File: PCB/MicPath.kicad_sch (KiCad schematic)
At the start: 53 parts, among them J301 NC3FAH, J302 Conn_01x02, J303 Conn_01x02, J304 Conn_01x02, J305 Conn_01x02, J306 NC3MAH, J307 NC3MAH, SW301 SW_SPST, SW302 SW_SPST, U301 THAT1512, U302 TMUX6236, U303 THAT1646, U304 THAT1646

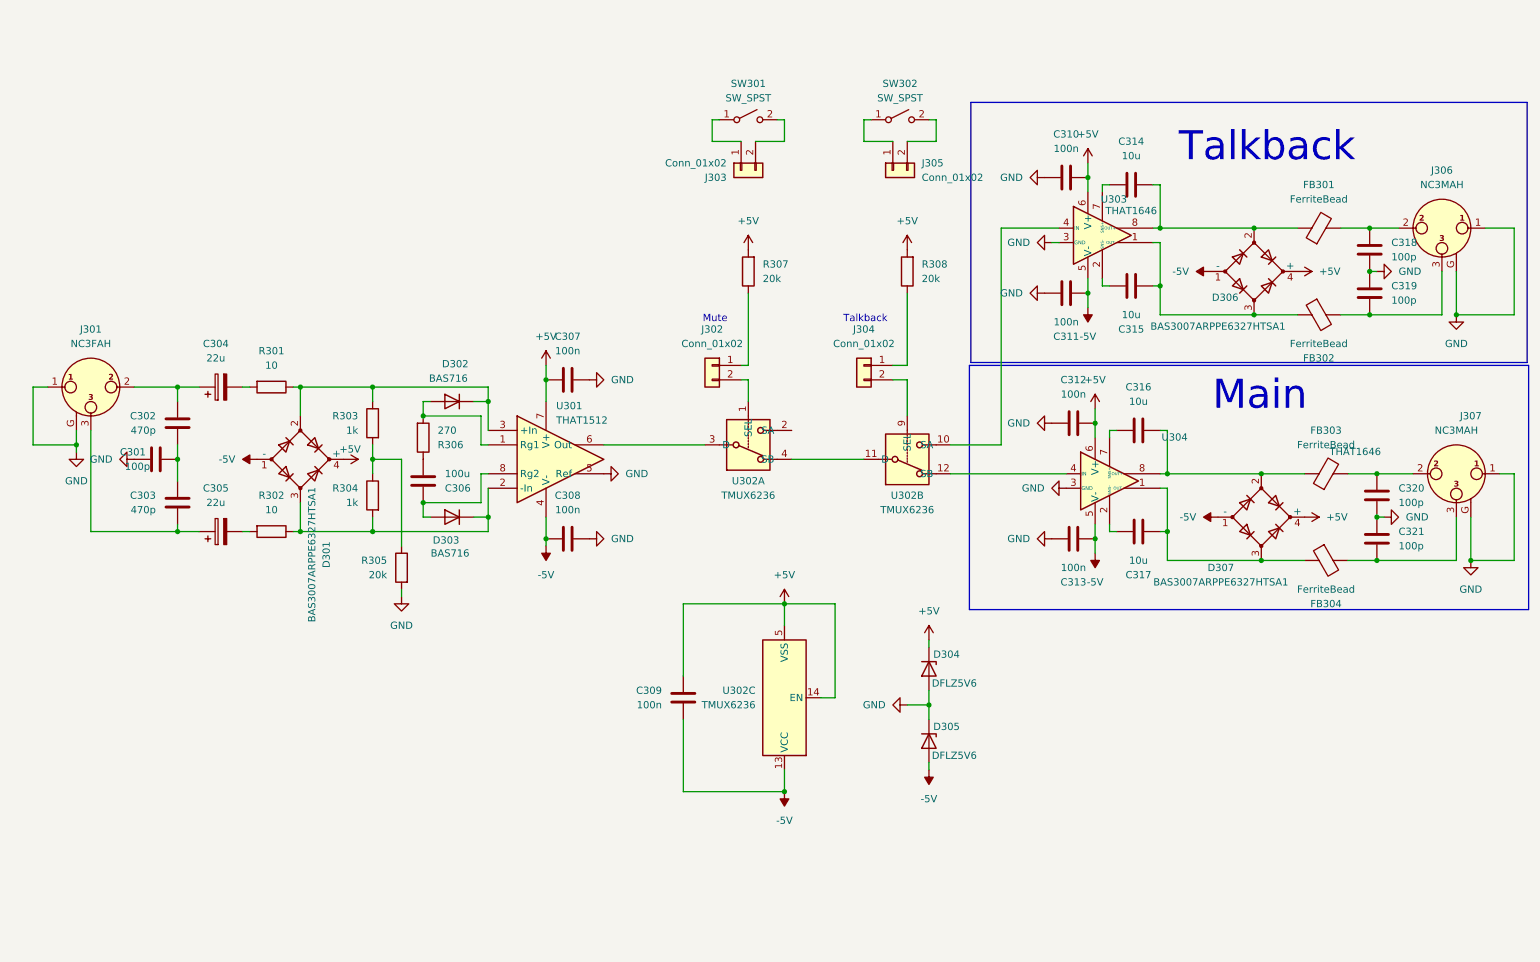
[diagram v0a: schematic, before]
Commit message: Wooooooo
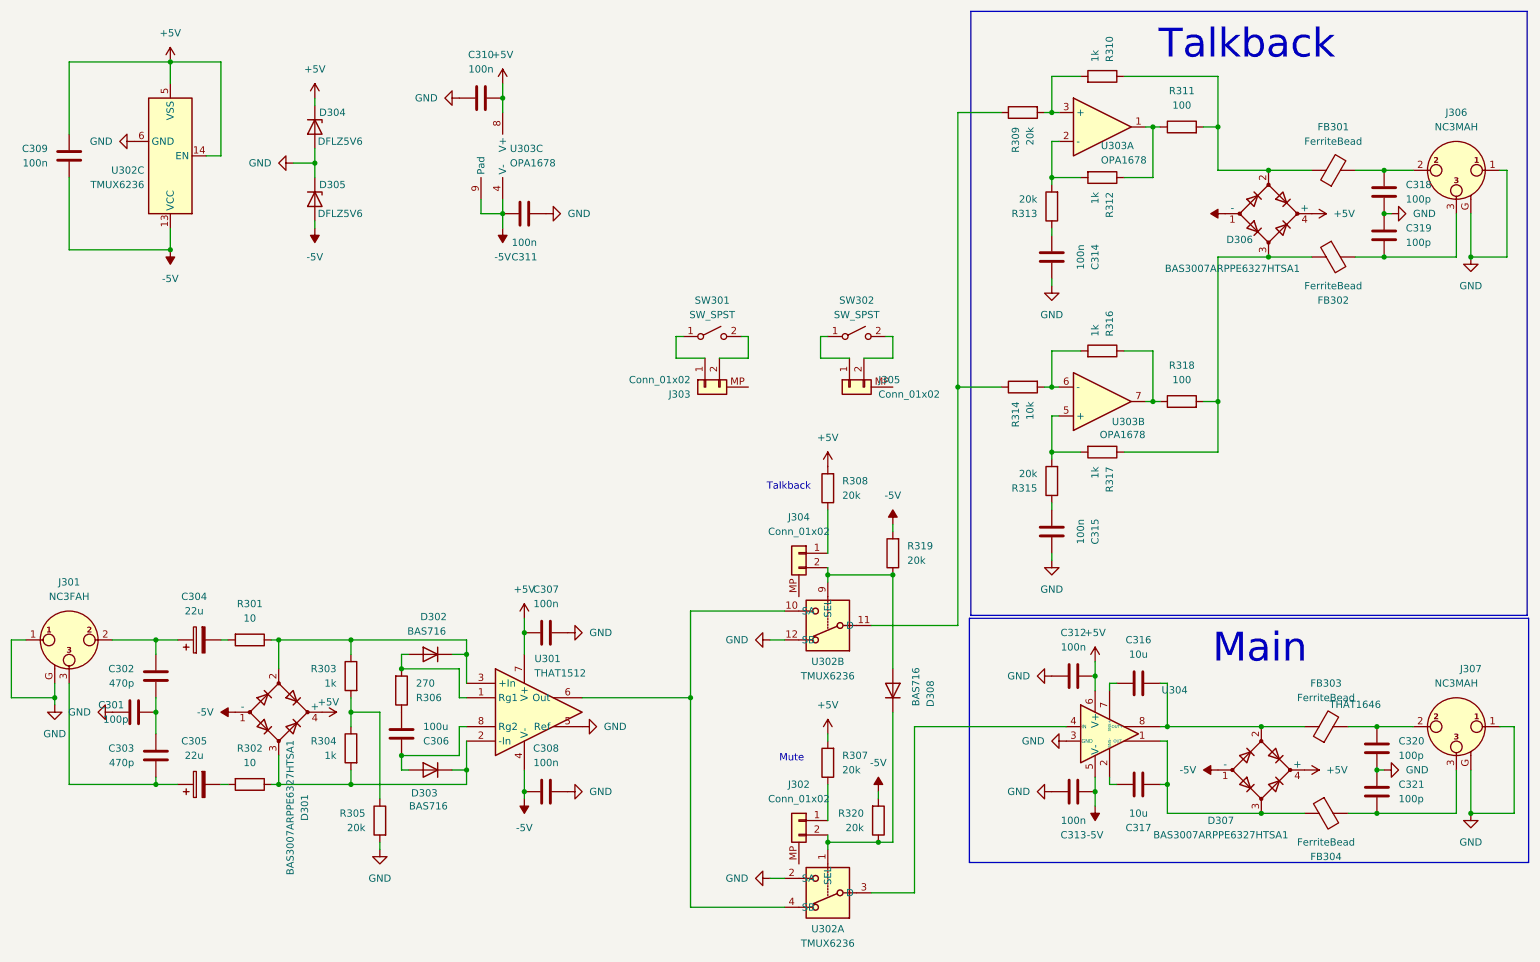
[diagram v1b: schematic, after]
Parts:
- removed U303: THAT1646, Package_SO:SO-8_3.9x4.9mm_P1.27mm, symbol STEVEannouncer:THAT1646
- added D308: BAS716, Diode_SMD:D_SOD-523, symbol Diode:1N4148WT
- added R309, R313, R315, R319, R320: 20k, Resistor_SMD:R_0402_1005Metric, symbol Device:R
- added R310, R312, R316, R317: 1k, Resistor_SMD:R_0402_1005Metric, symbol Device:R
- added R311, R318: 100, Resistor_SMD:R_0402_1005Metric, symbol Device:R
- added R314: 10k, Resistor_SMD:R_0402_1005Metric, symbol Device:R
- added U303: OPA1678, Package_SON:WSON-8-1EP_3x3mm_P0.5mm_EP1.2x2mm_ThermalVias, symbol STEVEannouncer:OPA1678
- C304, C305: footprint (none) -> Capacitor_SMD:CP_Elec_6.3x7.7; Mouser Part Number (none) -> 647-UCD1J220MCL1GS
- C306: footprint (none) -> Capacitor_SMD:C_1206_3216Metric; Mouser Part Number (none) -> 81-GRM31CR60J107KE8L
- C307, C308, C309, C310, C311, C312, C313: Mouser Part Number (none) -> 81-GRM155R62A104KE4D
- C314, C315: value 10u -> 100n; footprint (none) -> Capacitor_SMD:C_0402_1005Metric; Mouser Part Number (none) -> 81-GRM155R62A104KE4D
- C316, C317: footprint (none) -> Capacitor_SMD:C_0603_1608Metric; Mouser Part Number (none) -> 187-CL10A106KP8NNWC
- J302, J303, J304, J305: symbol Connector_Generic:Conn_01x02 -> STEVEannouncer:JST_B2B_PH
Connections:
- net +5V: now also U303.8 (V+)
- net -5V: now also R319.2, R320.2, U303.4 (V-), U303.9 (Pad)
- net GND: now also C314.1, C315.1, U302.12 (SB), U302.2 (SA), U302.6 (GND)
- net at J304.2 (Pin_2), U302.9 (SEL): now also D308.2 (A), R319.1
- net at J302.2 (Pin_2), U302.1 (SEL): now also D308.1 (K), R320.1
- net at D306.3, FB302.1: now also R317.1, R318.2; no longer C315.2
- net at U302.10 (SA): now also U301.6 (Out), U302.4 (SB)
- net at D306.2, FB301.1: now also R310.1, R311.2; no longer C314.2
- net at U302.11 (D): now also R309.1, R314.1; no longer U302.4 (SB)
- net at U304.4 (IN): now also U302.3 (D); no longer U302.12 (SB)
- new net: R315.2, R317.2, U303.5 (+)
- new net: R314.2, R316.2, U303.6 (-)
- new net: R316.1, R318.1, U303.7
- new net: C315.2, R315.1
- new net: R311.1, R312.1, U303.1
- new net: R312.2, R313.2, U303.2 (-)
- new net: R309.2, R310.2, U303.3 (+)
- new net: C314.2, R313.1
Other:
- moved on the sheet: C301, C302, C303, C304, C305, C306, C307, C308, C309, C310, C311, C312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
